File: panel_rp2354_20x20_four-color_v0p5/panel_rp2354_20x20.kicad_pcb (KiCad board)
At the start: 6 copper layers, 45 x 45 mm, 557 parts, among them J1 Conn_01x04, J2 Conn_01x05, J3 Conn_01x05, J4 Conn_01x05, J5 Conn_01x05, SW1 SW_Push, SW2 SW_Push, U1 APS6404L-3SQR, U10 UCC27517, U11 UCC27517, U12 UCC27517, U13 UCC27517, U14 UCC27517, U15 UCC27517, U16 UCC27517, U17 UCC27517, U18 UCC27517, U19 UCC27517, U2 RP2354B_80QFN, U20 UCC27517, U21 UCC27517, U22 UCC27517, U23 UCC27517, U24 UCC27517, U25 UCC27517, U26 UCC27517, U27 UCC27517, U28 UCC27517, U29 UCC27517, U3 UCC27517, U30 UCC27517, U31 UCC27517, U32 UCC27517, U33 UCC27517, U34 UCC27517, U35 UCC27517, U36 UCC27517, U37 UCC27517, U38 UCC27517, U39 UCC27517, U4 UCC27517, U40 UCC27517, U41 UCC27517, U42 UCC27517, U43 AP2112K-3.3, U5 UCC27517, U6 UCC27517, U7 UCC27517, U8 UCC27517, U9 UCC27517, Y1 ABM8-272-T3

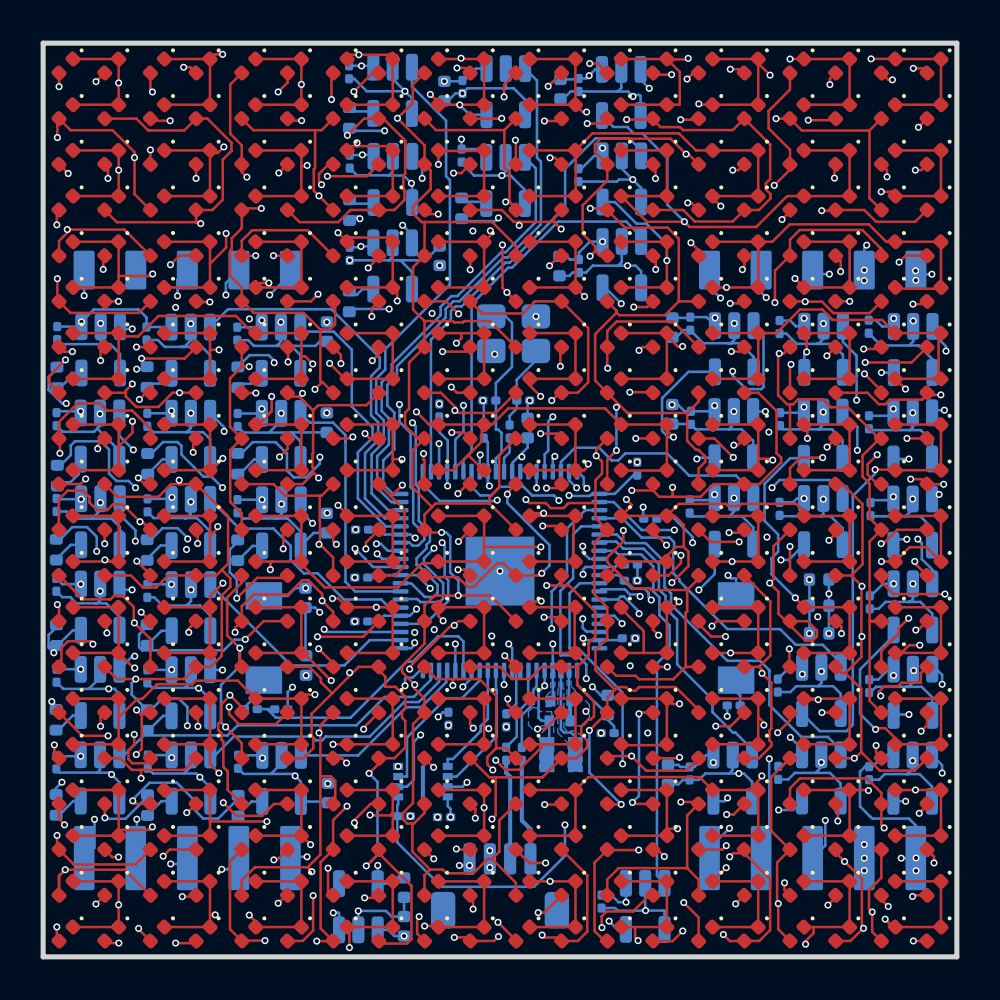
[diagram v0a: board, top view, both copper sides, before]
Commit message: manual cleanup
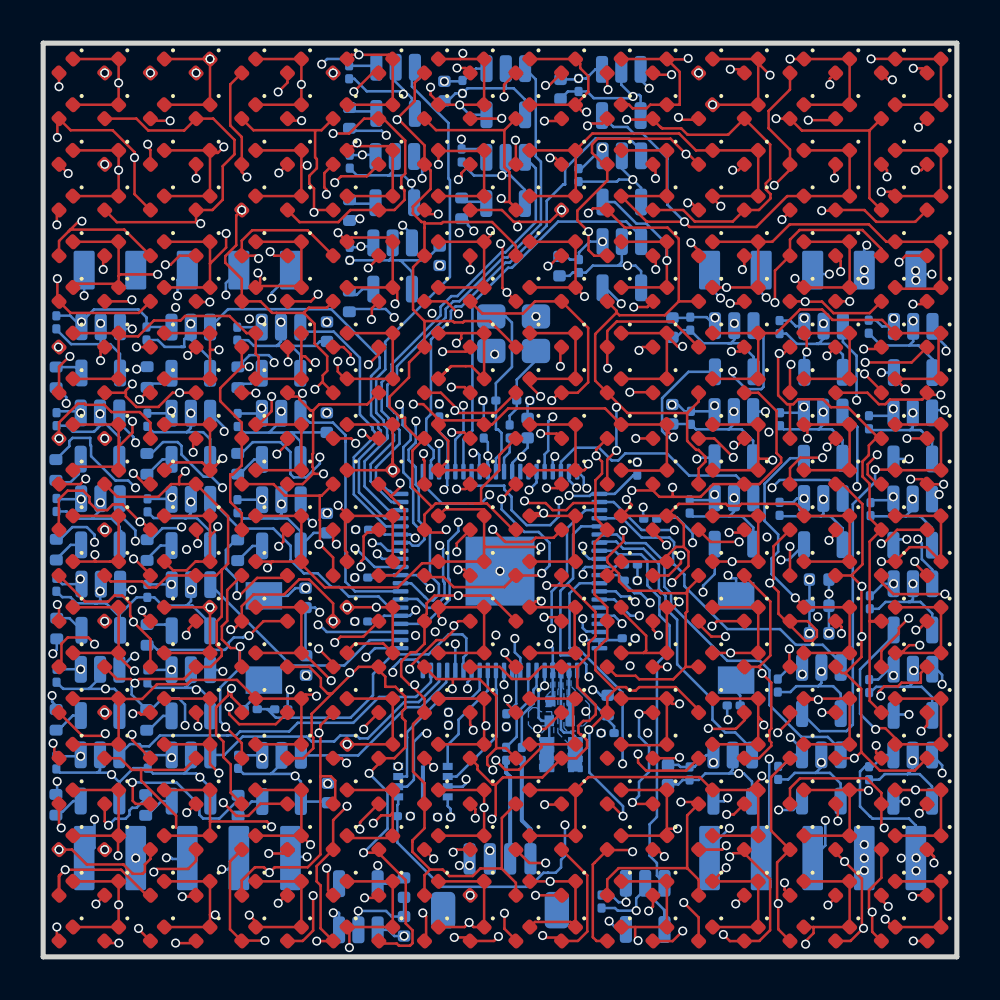
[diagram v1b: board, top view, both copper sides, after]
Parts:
- moved C32 0.53 mm to (50.6, 63.8)
- moved R15 0.33 mm to (50.7, 78.8), turned to -90 degrees
- moved R21 0.29 mm to (50.6, 71.0)
- moved U21 0.15 mm to (67.4, 52.3)
- moved U17 0.10 mm to (67.3, 56.7)
- moved R10 0.09 mm to (55.0, 87.5)
- turned R22 to -90 degrees
- turned R14 to -90 degrees
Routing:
- net GND: track 260.3 -> 273.0 mm
- net Net-(D100-A): track 115.5 -> 123.4 mm
- net +5V: track 100.4 -> 106.6 mm, vias 57 -> 56
- net Net-(D101-A): track 125.8 -> 131.1 mm
- net /drivers/ROW_06: track 92.2 -> 97.0 mm
- net Net-(D181-A): track 142.5 -> 146.9 mm
- net Net-(D1-A): track 110.9 -> 114.5 mm, vias 17 -> 16
- net Net-(D141-A): track 125.9 -> 129.4 mm
- net Net-(D221-A): track 130.2 -> 133.4 mm
- net Net-(D261-A): track 144.7 -> 141.6 mm
- net Net-(D161-A): track 113.9 -> 117.0 mm
- net Net-(D41-A): track 114.5 -> 117.1 mm
- net Net-(D201-A): track 125.1 -> 127.7 mm
- net Net-(D241-A): track 140.0 -> 142.3 mm
- net +1V1: track 37.9 -> 40.1 mm
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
